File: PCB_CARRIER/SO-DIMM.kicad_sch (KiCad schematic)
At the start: 1 part, among them J1 SODIMM-260_Split

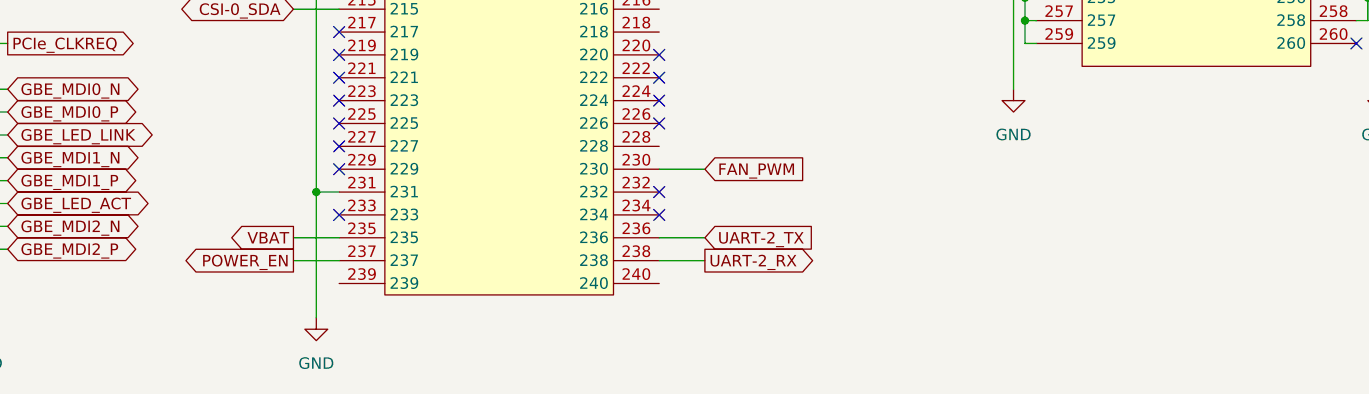
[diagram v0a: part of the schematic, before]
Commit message: added sleep/wake and sys_reset
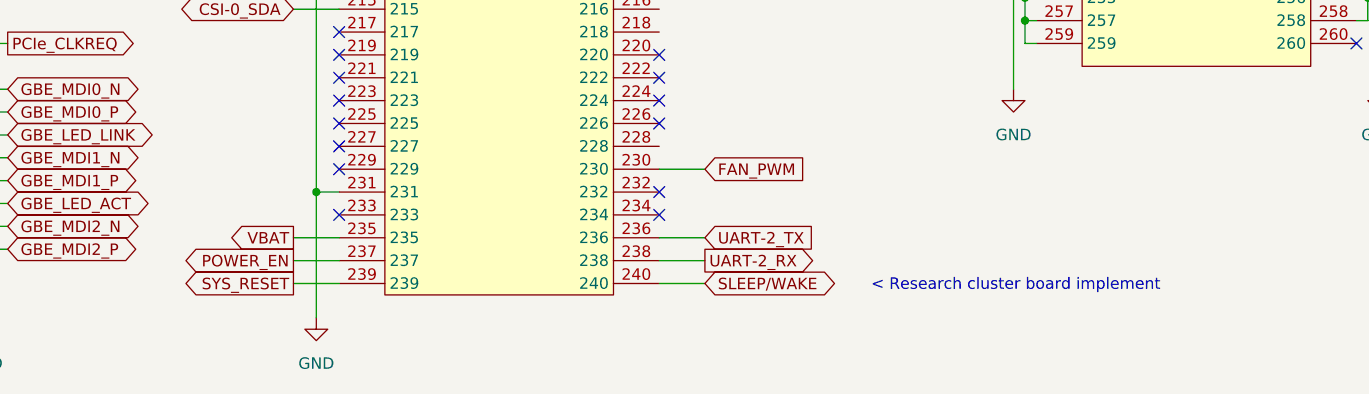
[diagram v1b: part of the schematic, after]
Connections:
- net SYS_RESET: now reaches J1.239
- net SLEEP/WAKE: now reaches J1.240
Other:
- note added: "< Research cluster board implement"
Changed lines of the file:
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@@
 		)
 	)
+	(text "< Research cluster board implement"
+		(exclude_from_sim no)
+		(at 232.664 203.454 0)
+		(effects
+			(font
+				(size 1.27 1.27)
+			)
+		)
+	)
 	(text "< Second camera?"
 		(exclude_from_sim no)
@@
 	(wire
 		(pts
+			(xy 152.4 203.2) (xy 157.48 203.2)
+		)
+		(stroke
+			(width 0)
+			(type default)
+		)
+	)
+	(wire
+		(pts
 			(xy 120.65 96.52) (xy 115.57 96.52)
 		)
@@
 	(wire
 		(pts
+			(xy 198.12 203.2) (xy 193.04 203.2)
+		)
+		(stroke
+			(width 0)
+			(type default)
+		)
+	)
+	(wire
+		(pts
 			(xy 152.4 160.02) (xy 157.48 160.02)
 		)
@@
 			(effects
 				(font
+					(size 1.27 1.27)
+				)
+				(justify left)
+				(hide yes)
+			)
+		)
+	)
+	(global_label "SYS_RESET"
+		(shape output)
+		(at 152.4 203.2 180)
+		(fields_autoplaced yes)
+		(effects
+			(font
+				(size 1.27 1.27)
+			)
+			(justify right)
+		)
+		(property "Intersheetrefs" "${INTERSHEET_REFS}"
+			(at 139.0994 203.2 0)
+			(effects
+				(font
+					(size 1.27 1.27)
+				)
+				(justify right)
+				(hide yes)
+			)
+		)
+	)
+	(global_label "SLEEP{slash}WAKE"
+		(shape bidirectional)
+		(at 198.12 203.2 0)
+		(fields_autoplaced yes)
+		(effects
+			(font
+				(size 1.27 1.27)
+			)
+			(justify left)
+		)
+		(property "Intersheetrefs" "${INTERSHEET_REFS}"
+			(at 214.3114 203.2 0)
+			(effects
+				(font

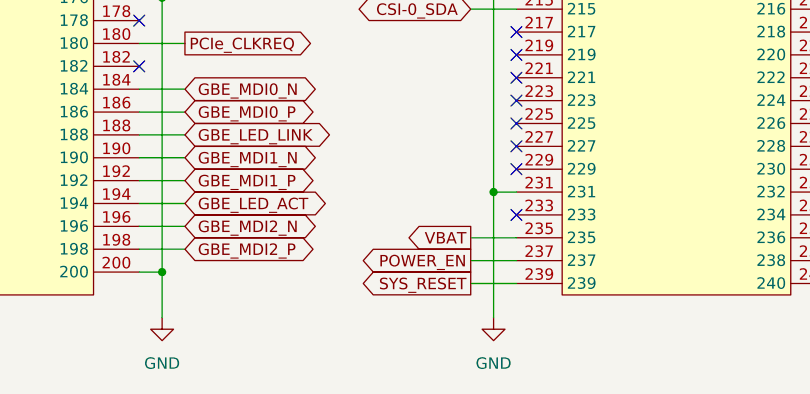
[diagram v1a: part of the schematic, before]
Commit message: added the NMOS for the PWR state
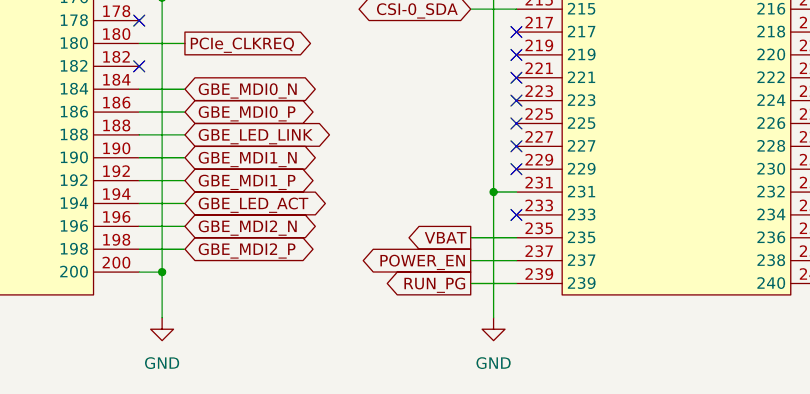
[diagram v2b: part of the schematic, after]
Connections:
- net SYS_RESET renamed RUN_PG
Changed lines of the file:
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@@
+		)
+	)
+	(global_label "RUN_PG"
+		(shape output)
+		(at 152.4 203.2 180)
+		(fields_autoplaced yes)
+		(effects
+			(font
+				(size 1.27 1.27)
+			)
+			(justify right)
+		)
+		(property "Intersheetrefs" "${INTERSHEET_REFS}"
+			(at 141.8811 203.2 0)
+			(effects
+				(font
+					(size 1.27 1.27)
+				)
+				(justify right)
+				(hide yes)
+			)
 		)
 	)
@@
 				(hide yes)
 			)
-		)
-	)
-	(global_label "SYS_RESET"
-		(shape output)
-		(at 152.4 203.2 180)
-		(fields_autoplaced yes)
-		(effects
-			(font
-				(size 1.27 1.27)
-			)
-			(justify right)
-		)
-		(property "Intersheetrefs" "${INTERSHEET_REFS}"
-			(at 139.0994 203.2 0)
-			(effects
-				(font
-					(size 1.27 1.27)
-				)
-				(justify right)
-				(hide yes)
-			)

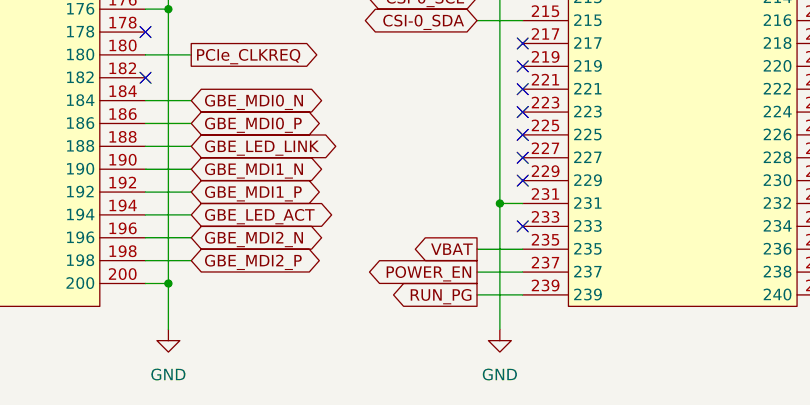
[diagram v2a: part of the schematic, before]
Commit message: adding NMOS for the POWER
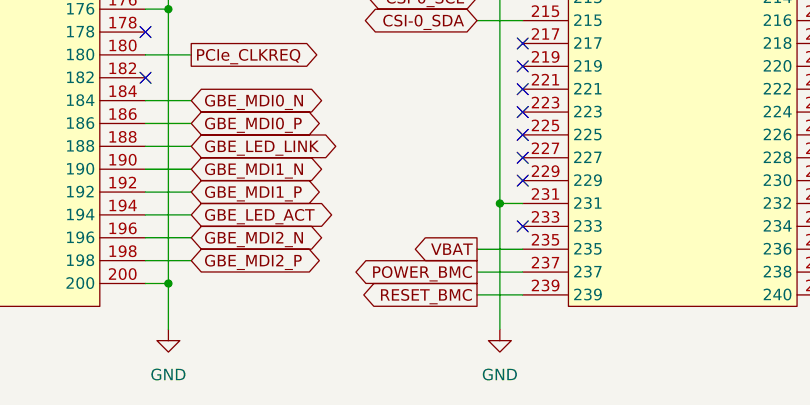
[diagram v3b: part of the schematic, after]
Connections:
- net POWER_EN renamed POWER_BMC
- net RUN_PG renamed RESET_BMC
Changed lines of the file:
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@@
 		)
 	)
-	(global_label "POWER_EN"
+	(global_label "POWER_BMC"
 		(shape output)
 		(at 152.4 200.66 180)
@@
 		)
 		(property "Intersheetrefs" "${INTERSHEET_REFS}"
-			(at 139.4017 200.66 0)
+			(at 137.8898 200.66 0)
 			(effects
 				(font
@@
 		)
 	)
-	(global_label "RUN_PG"
+	(global_label "RESET_BMC"
 		(shape output)
 		(at 152.4 203.2 180)
@@
 		)
 		(property "Intersheetrefs" "${INTERSHEET_REFS}"
-			(at 141.8811 203.2 0)
-			(effects
-				(font
+			(at 138.6156 203.2 0)
+			(effects
+				(font

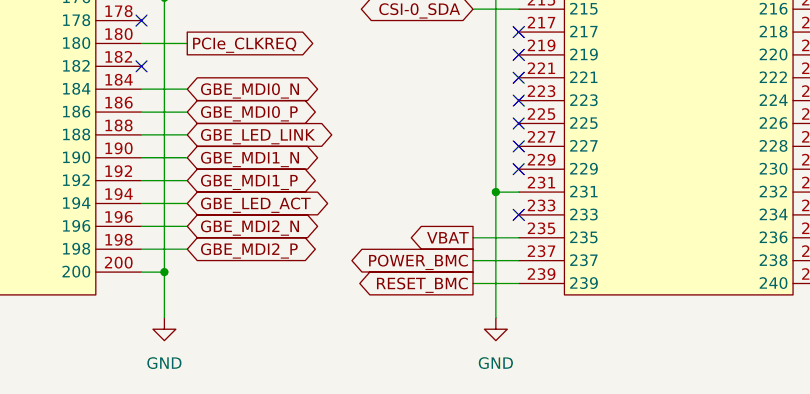
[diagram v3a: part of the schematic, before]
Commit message: added system reset
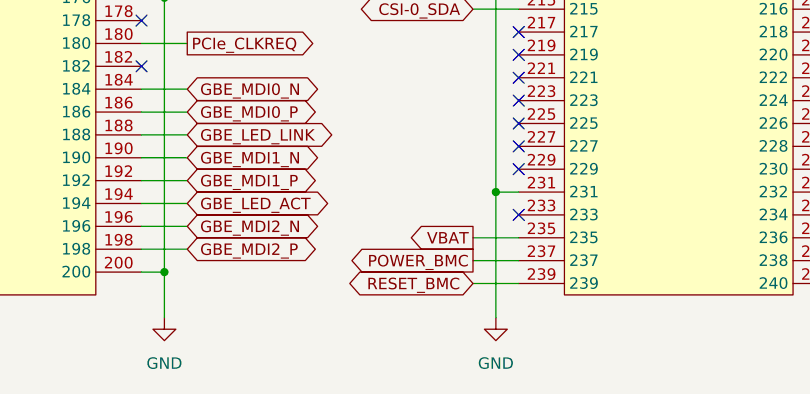
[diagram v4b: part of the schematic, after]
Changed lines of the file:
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@@
 	)
 	(global_label "RESET_BMC"
-		(shape output)
+		(shape bidirectional)
 		(at 152.4 203.2 180)
 		(fields_autoplaced yes)
@@
 		)
 		(property "Intersheetrefs" "${INTERSHEET_REFS}"
-			(at 138.6156 203.2 0)
+			(at 137.5996 203.2 0)
 			(effects
 				(font

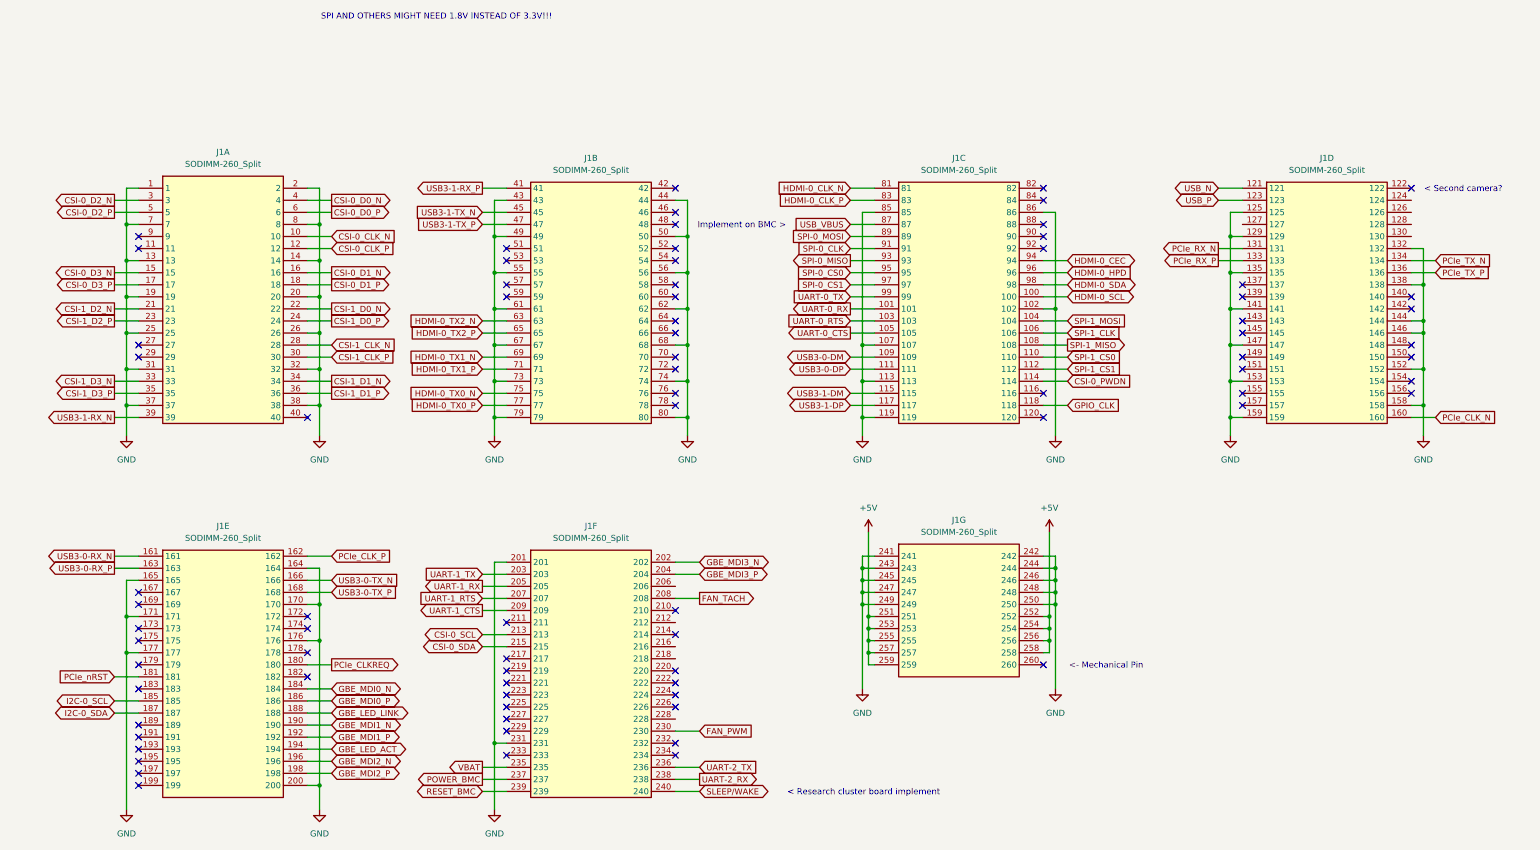
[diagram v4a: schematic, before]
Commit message: adding shutdown req
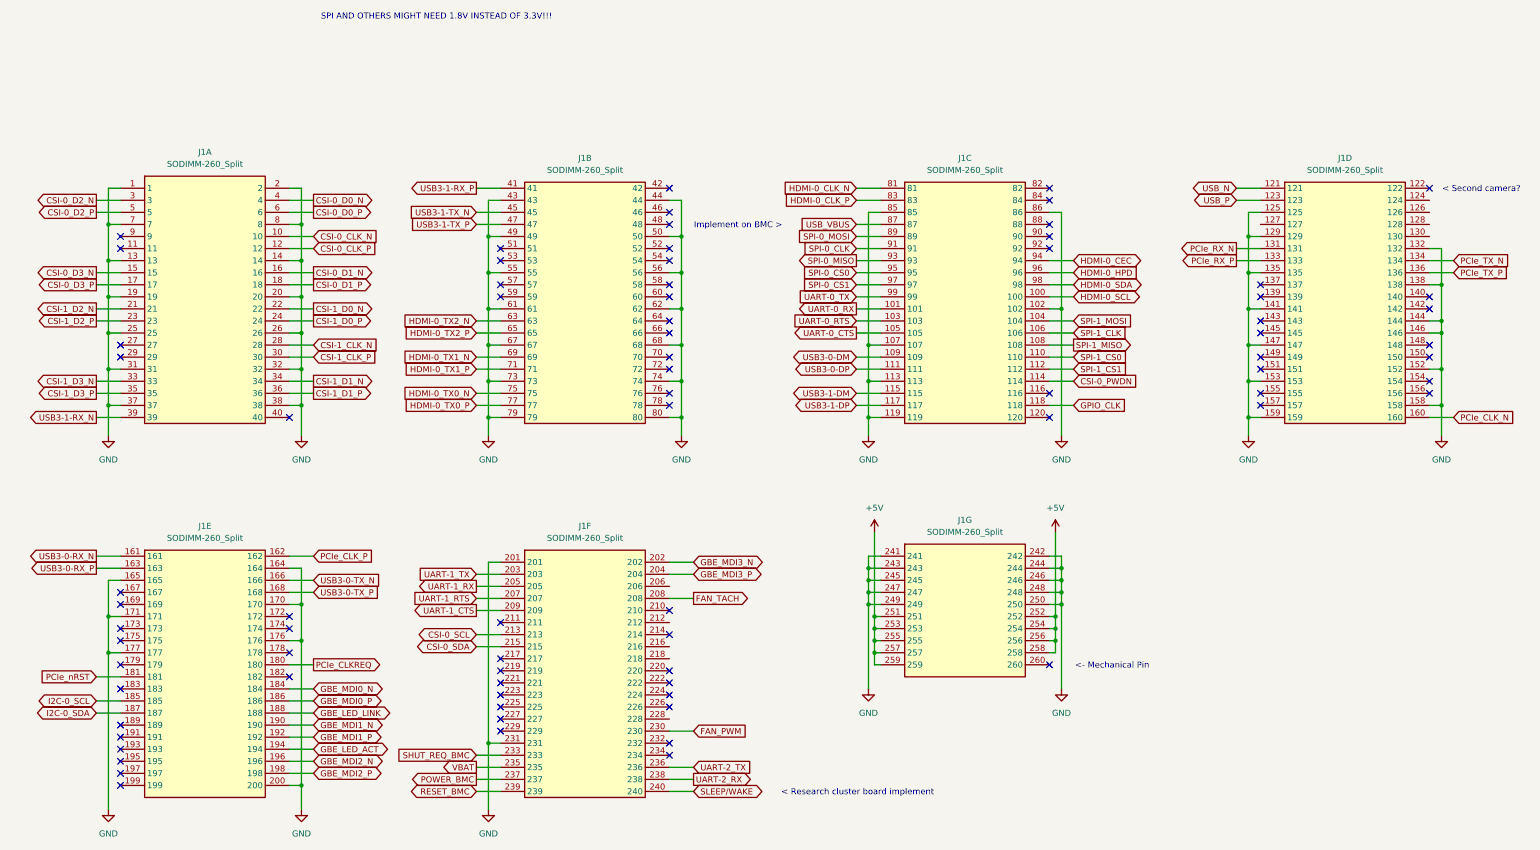
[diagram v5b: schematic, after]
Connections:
- net SHUT_REQ_BMC: now reaches J1.233
- no-connect marks 78 -> 77
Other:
- moved on the sheet: J1A, J1B, J1C, J1D, J1E, J1F, J1G
